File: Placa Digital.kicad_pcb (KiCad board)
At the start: 2 copper layers, 60 x 80 mm, 23 parts, among them J1 Entradas / Salidas, Q1 BC548, Q2 BC548, U1 EC11_Module, U2 Alimentación, U3 ST7920_Display, U4 10K, U5 MX1A-11NN, U6 MX1A-11NN, U7 MX1A-11NN

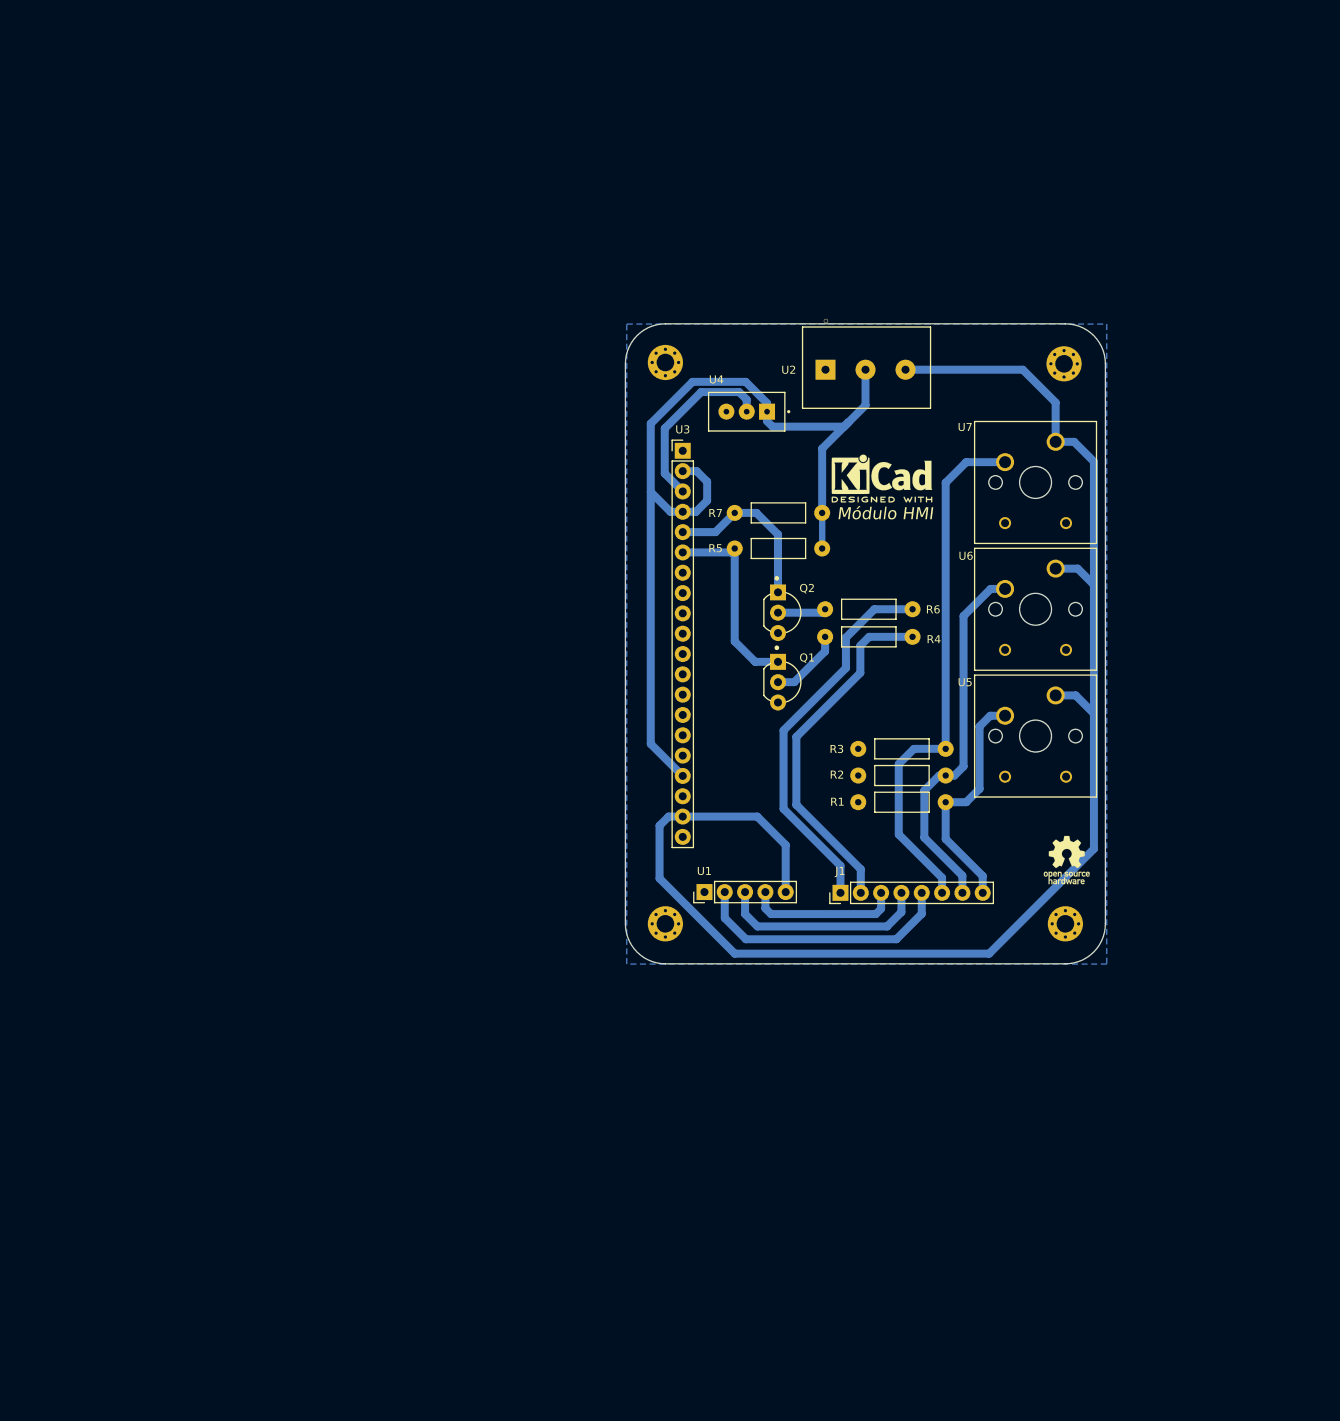
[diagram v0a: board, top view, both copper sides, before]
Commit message: Last version
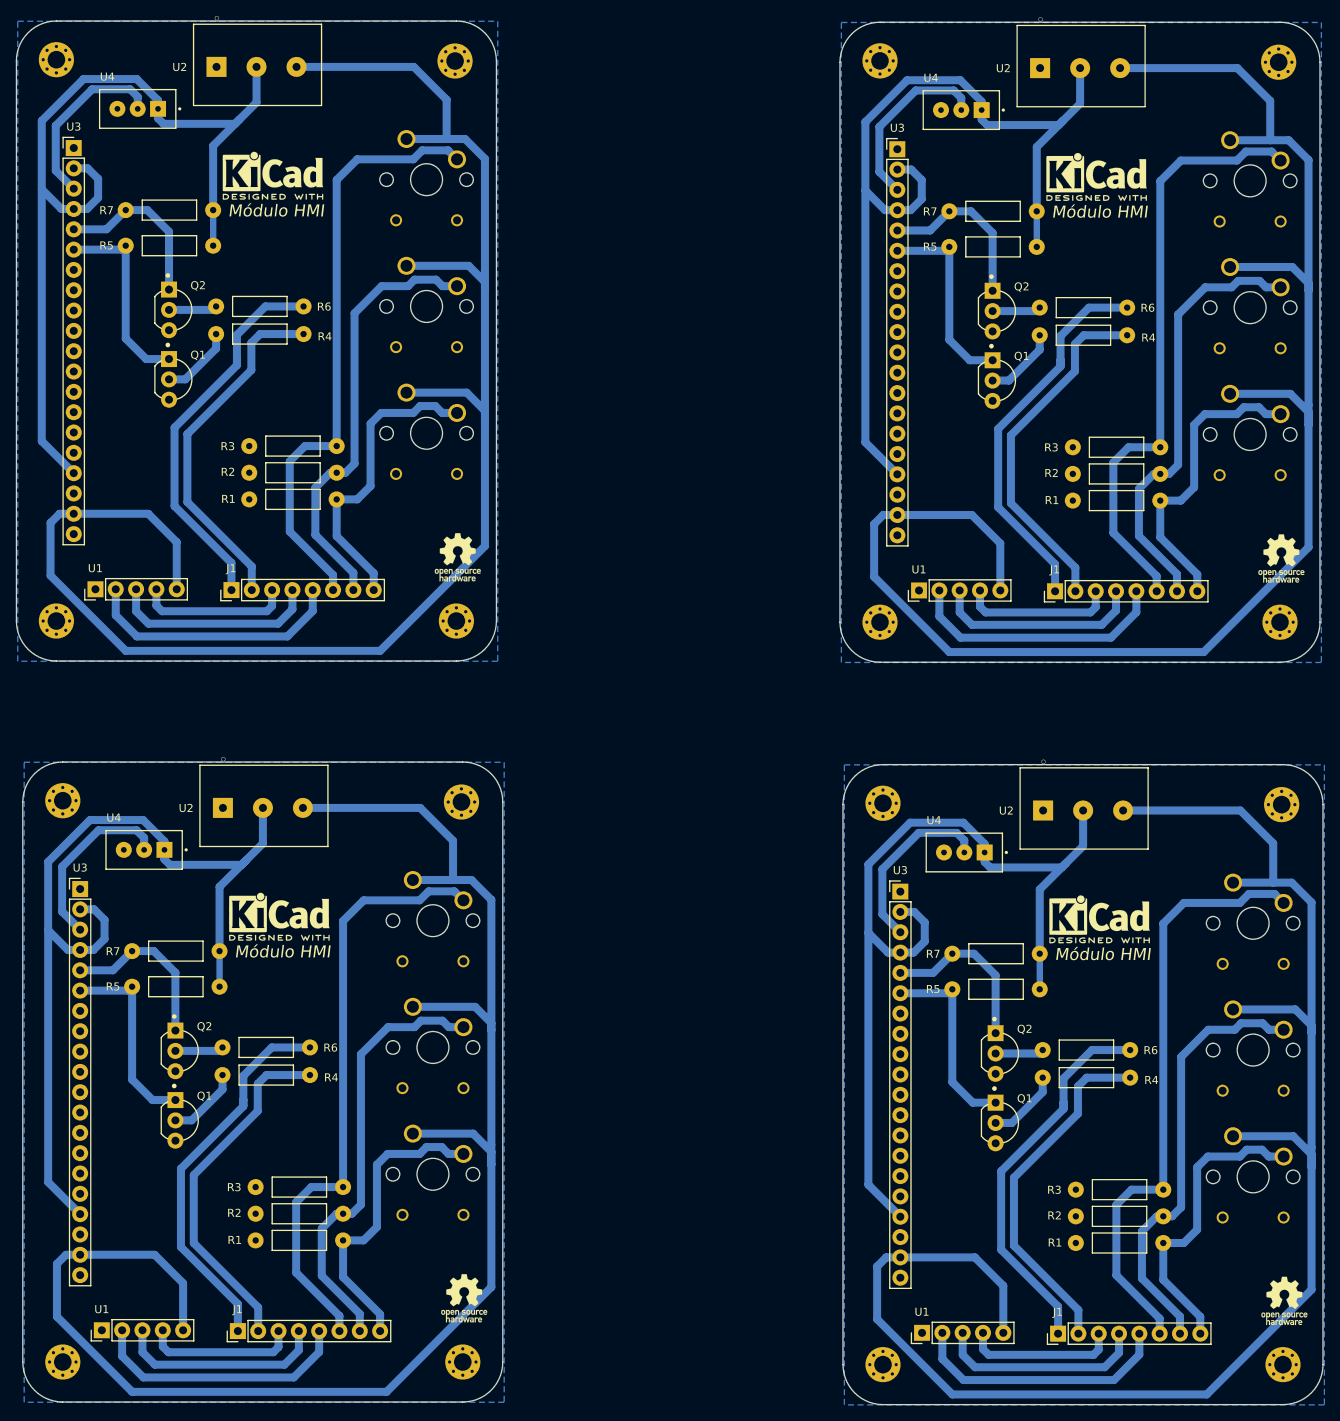
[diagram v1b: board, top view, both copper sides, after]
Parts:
- added H1: MountingHole, MountingHole:MountingHole_2.2mm_M2_Pad_Via, F.Cu at (142.3, 26.4)
- added H1: MountingHole, MountingHole:MountingHole_2.2mm_M2_Pad_Via, F.Cu at (40.1, 118.9)
- added H1: MountingHole, MountingHole:MountingHole_2.2mm_M2_Pad_Via, F.Cu at (142.6, 119.2)
- added H2: MountingHole, MountingHole:MountingHole_2.2mm_M2_Pad_Via, F.Cu at (90.0, 119.1)
- added H2: MountingHole, MountingHole:MountingHole_2.2mm_M2_Pad_Via, F.Cu at (192.1, 26.6)
- added H2: MountingHole, MountingHole:MountingHole_2.2mm_M2_Pad_Via, F.Cu at (192.5, 119.4)
- added H3: MountingHole, MountingHole:MountingHole_2.2mm_M2_Pad_Via, F.Cu at (192.6, 189.4)
- added H3: MountingHole, MountingHole:MountingHole_2.2mm_M2_Pad_Via, F.Cu at (192.3, 96.6)
- added H3: MountingHole, MountingHole:MountingHole_2.2mm_M2_Pad_Via, F.Cu at (90.1, 189.1)
- added H4: MountingHole, MountingHole:MountingHole_2.2mm_M2_Pad_Via, F.Cu at (142.6, 189.4)
- added H4: MountingHole, MountingHole:MountingHole_2.2mm_M2_Pad_Via, F.Cu at (142.3, 96.6)
- added H4: MountingHole, MountingHole:MountingHole_2.2mm_M2_Pad_Via, F.Cu at (40.1, 189.1)
- added J1: Entradas / Salidas, Connector_PinHeader_2.54mm:PinHeader_1x08_P2.54mm_Vertical, F.Cu at (62.0, 185.2)
- added J1: Entradas / Salidas, Connector_PinHeader_2.54mm:PinHeader_1x08_P2.54mm_Vertical, F.Cu at (164.2, 92.7)
- added J1: Entradas / Salidas, Connector_PinHeader_2.54mm:PinHeader_1x08_P2.54mm_Vertical, F.Cu at (164.5, 185.5)
- added Q1: BC548, CEDCp:BC548, F.Cu at (157.6, 159.2)
- added Q1: BC548, CEDCp:BC548, F.Cu at (157.2, 66.4)
- added Q1: BC548, CEDCp:BC548, F.Cu at (55.1, 158.9)
- added Q2: BC548, CEDCp:BC548, F.Cu at (55.1, 150.2)
- added Q2: BC548, CEDCp:BC548, F.Cu at (157.6, 150.5)
- added Q2: BC548, CEDCp:BC548, F.Cu at (157.2, 57.7)
- added R1: 10k, CEDCp:Resistencia_0,25W, F.Cu at (172.2, 174.2)
- added R1: 10k, CEDCp:Resistencia_0,25W, F.Cu at (171.8, 81.4)
- added R1: 10k, CEDCp:Resistencia_0,25W, F.Cu at (69.7, 173.9)
- added R2: 10k, CEDCp:Resistencia_0,25W, F.Cu at (171.8, 78.1)
- added R2: 10k, CEDCp:Resistencia_0,25W, F.Cu at (69.7, 170.5)
- added R2: 10k, CEDCp:Resistencia_0,25W, F.Cu at (172.2, 170.9)
- added R3: 10k, CEDCp:Resistencia_0,25W, F.Cu at (69.7, 167.2)
- added R3: 10k, CEDCp:Resistencia_0,25W, F.Cu at (172.2, 167.5)
- added R3: 10k, CEDCp:Resistencia_0,25W, F.Cu at (171.8, 74.7)
- added R4: 2k7, CEDCp:Resistencia_0,25W, F.Cu at (168.1, 153.5)
- added R4: 2k7, CEDCp:Resistencia_0,25W, F.Cu at (167.7, 60.7)
- added R4: 2k7, CEDCp:Resistencia_0,25W, F.Cu at (65.6, 153.2)
- added R5: 1k, CEDCp:Resistencia_0,25W, F.Cu at (54.3, 142.1)
- added R5: 1k, CEDCp:Resistencia_0,25W, F.Cu at (156.8, 142.5)
- added R5: 1k, CEDCp:Resistencia_0,25W, F.Cu at (156.4, 49.7)
- added R6: 2k7, CEDCp:Resistencia_0,25W, F.Cu at (167.7, 57.3)
- added R6: 2k7, CEDCp:Resistencia_0,25W, F.Cu at (65.6, 149.7)
- added R6: 2k7, CEDCp:Resistencia_0,25W, F.Cu at (168.1, 150.1)
- added R7: 1k, CEDCp:Resistencia_0,25W, F.Cu at (156.4, 45.2)
- added R7: 1k, CEDCp:Resistencia_0,25W, F.Cu at (54.3, 137.7)
- added R7: 1k, CEDCp:Resistencia_0,25W, F.Cu at (156.8, 138.0)
- added REF**: KiCad-Logo2_5mm_SilkScreen, Symbol:KiCad-Logo2_5mm_SilkScreen, F.Cu at (67.2, 133.4)
- added REF**: OSHW-Logo_5.7x6mm_SilkScreen, Symbol:OSHW-Logo_5.7x6mm_SilkScreen, F.Cu at (90.3, 181.1)
- added REF**: KiCad-Logo2_5mm_SilkScreen, Symbol:KiCad-Logo2_5mm_SilkScreen, F.Cu at (169.3, 40.9)
- added REF**: KiCad-Logo2_5mm_SilkScreen, Symbol:KiCad-Logo2_5mm_SilkScreen, F.Cu at (169.7, 133.7)
- added REF**: OSHW-Logo_5.7x6mm_SilkScreen, Symbol:OSHW-Logo_5.7x6mm_SilkScreen, F.Cu at (192.4, 88.6)
- added REF**: OSHW-Logo_5.7x6mm_SilkScreen, Symbol:OSHW-Logo_5.7x6mm_SilkScreen, F.Cu at (192.8, 181.4)
- added U1: EC11_Module, Connector_PinHeader_2.54mm:PinHeader_1x05_P2.54mm_Vertical, F.Cu at (45.0, 185.1)
- added U1: EC11_Module, Connector_PinHeader_2.54mm:PinHeader_1x05_P2.54mm_Vertical, F.Cu at (147.2, 92.6)
- added U1: EC11_Module, Connector_PinHeader_2.54mm:PinHeader_1x05_P2.54mm_Vertical, F.Cu at (147.5, 185.4)
- added U2: Alimentación, CEDCp:Bornera_1x3, F.Cu at (167.7, 120.1)
- added U2: Alimentación, CEDCp:Bornera_1x3, F.Cu at (65.1, 119.8)
- added U2: Alimentación, CEDCp:Bornera_1x3, F.Cu at (167.3, 27.3)
- added U3: ST7920_Display, Connector_PinHeader_2.54mm:PinHeader_1x20_P2.54mm_Vertical, F.Cu at (144.4, 37.5)
- added U3: ST7920_Display, Connector_PinHeader_2.54mm:PinHeader_1x20_P2.54mm_Vertical, F.Cu at (42.3, 129.9)
- added U3: ST7920_Display, Connector_PinHeader_2.54mm:PinHeader_1x20_P2.54mm_Vertical, F.Cu at (144.8, 130.3)
- added U4: 10K, CEDCp:Preset_Multivueltas_Vertical, F.Cu at (152.4, 32.6)
- added U4: 10K, CEDCp:Preset_Multivueltas_Vertical, F.Cu at (50.3, 125.0)
- added U4: 10K, CEDCp:Preset_Multivueltas_Vertical, F.Cu at (152.8, 125.4)
- added U5: MX1A-11NN, CEDCp:CHERRY_MX1A-11NN_SWITCH, B.Cu at (188.5, 73.1)
- added U5: MX1A-11NN, CEDCp:CHERRY_MX1A-11NN_SWITCH, B.Cu at (86.4, 165.6)
- added U5: MX1A-11NN, CEDCp:CHERRY_MX1A-11NN_SWITCH, B.Cu at (188.9, 165.9)
- added U6: MX1A-11NN, CEDCp:CHERRY_MX1A-11NN_SWITCH, B.Cu at (188.5, 57.3)
- added U6: MX1A-11NN, CEDCp:CHERRY_MX1A-11NN_SWITCH, B.Cu at (86.4, 149.7)
- added U6: MX1A-11NN, CEDCp:CHERRY_MX1A-11NN_SWITCH, B.Cu at (188.9, 150.1)
- added U7: MX1A-11NN, CEDCp:CHERRY_MX1A-11NN_SWITCH, B.Cu at (188.5, 41.4)
- added U7: MX1A-11NN, CEDCp:CHERRY_MX1A-11NN_SWITCH, B.Cu at (188.9, 134.2)
- added U7: MX1A-11NN, CEDCp:CHERRY_MX1A-11NN_SWITCH, B.Cu at (86.4, 133.9)
- U5, U6, U7: moved to B.Cu
- moved R4 85.0 mm to (64.8, 60.6)
- moved R6 85.0 mm to (64.8, 57.1)
- moved U5 85.0 mm to (85.6, 73.0), turned to 180 degrees
- moved U6 85.0 mm to (85.6, 57.1), turned to 180 degrees
- moved U7 85.0 mm to (85.6, 41.3), turned to 180 degrees
- moved H1 85.0 mm to (39.3, 26.3)
- moved H3 85.0 mm to (89.3, 96.4)
- moved H4 85.0 mm to (39.3, 96.4)
- moved J1 85.0 mm to (61.2, 92.6)
- moved Q1 85.0 mm to (54.3, 66.2)
- moved Q2 85.0 mm to (54.3, 57.5)
- moved R1 85.0 mm to (68.9, 81.2)
- moved R2 85.0 mm to (68.9, 77.9)
- moved R3 85.0 mm to (68.9, 74.6)
- moved R5 85.0 mm to (53.5, 49.5)
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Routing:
- net +3V3: track 187.3 -> 809.3 mm
- net +5V: track 158.8 -> 635.3 mm
- net /toMicroC_Button3: track 66.8 -> 301.2 mm
- net /toMicroC_Button2: track 46.3 -> 218.4 mm
- net /fromMicroC_DisplaySID: track 48.6 -> 194.3 mm
- net /fromMicroC_DisplaySCLK: track 44.5 -> 178.1 mm
- net /toMicroC_Button1: track 29.7 -> 152.2 mm
- net Net-(Q1-Pad1): track 36.4 -> 145.8 mm
- net /toMicroC_EncoderSignalA: track 32.9 -> 131.7 mm
- net Net-(U3-Pad3): track 28.5 -> 113.9 mm
- net /toMicroC_EncoderSignalB: track 26.1 -> 104.3 mm
- net Net-(Q2-Pad1): track 21.3 -> 85.1 mm
- net /toMicroC_EncoderButton: track 19.1 -> 76.3 mm
- net Net-(Q1-Pad2): track 9.29 -> 37.2 mm
- net Net-(Q2-Pad2): track 6.07 -> 24.3 mm
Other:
- board size 60 x 80 mm -> 163.3 x 173 mm
